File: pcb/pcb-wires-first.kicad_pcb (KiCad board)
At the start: 2 copper layers, 24 x 28.5 mm, 13 parts, among them J3 Conn_01x04, J4 Conn_01x06, SW1 SW_Push, SW2 SW_Push, U1 SLG47115V

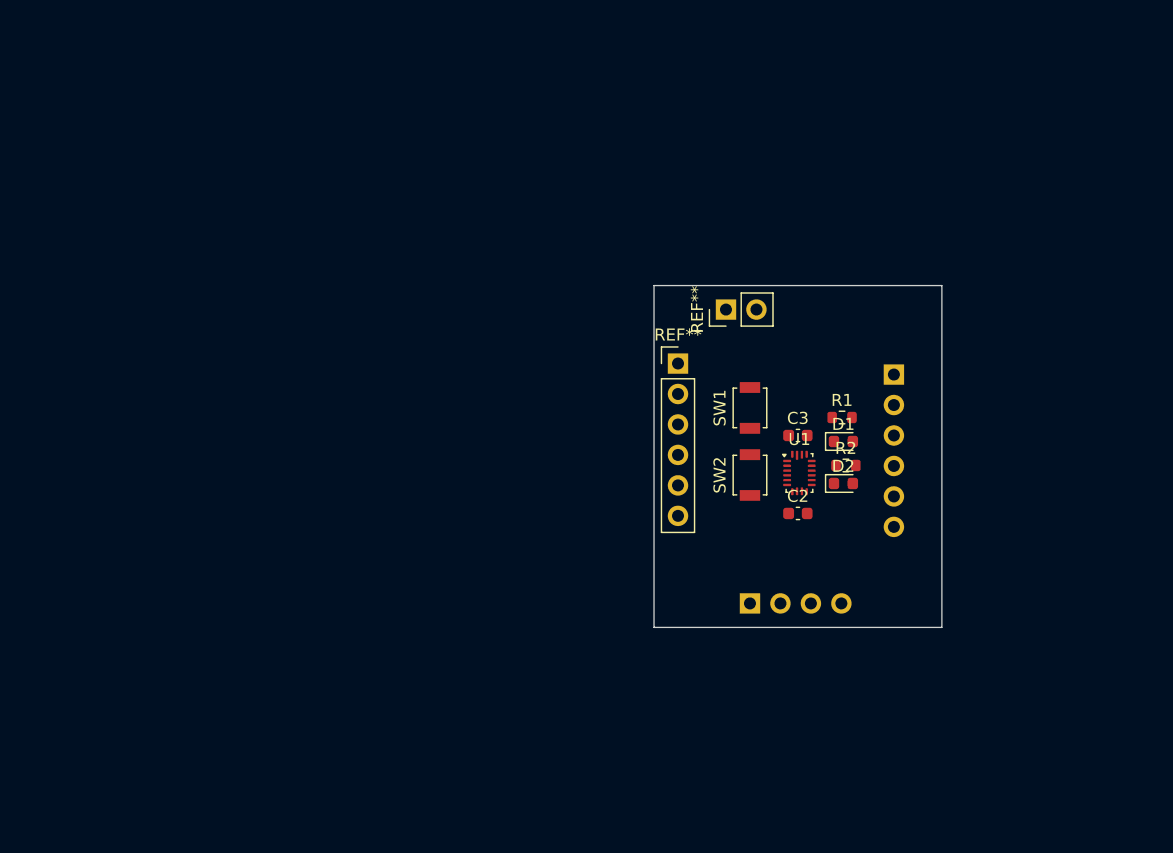
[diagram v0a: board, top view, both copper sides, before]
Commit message: Drafting the board.
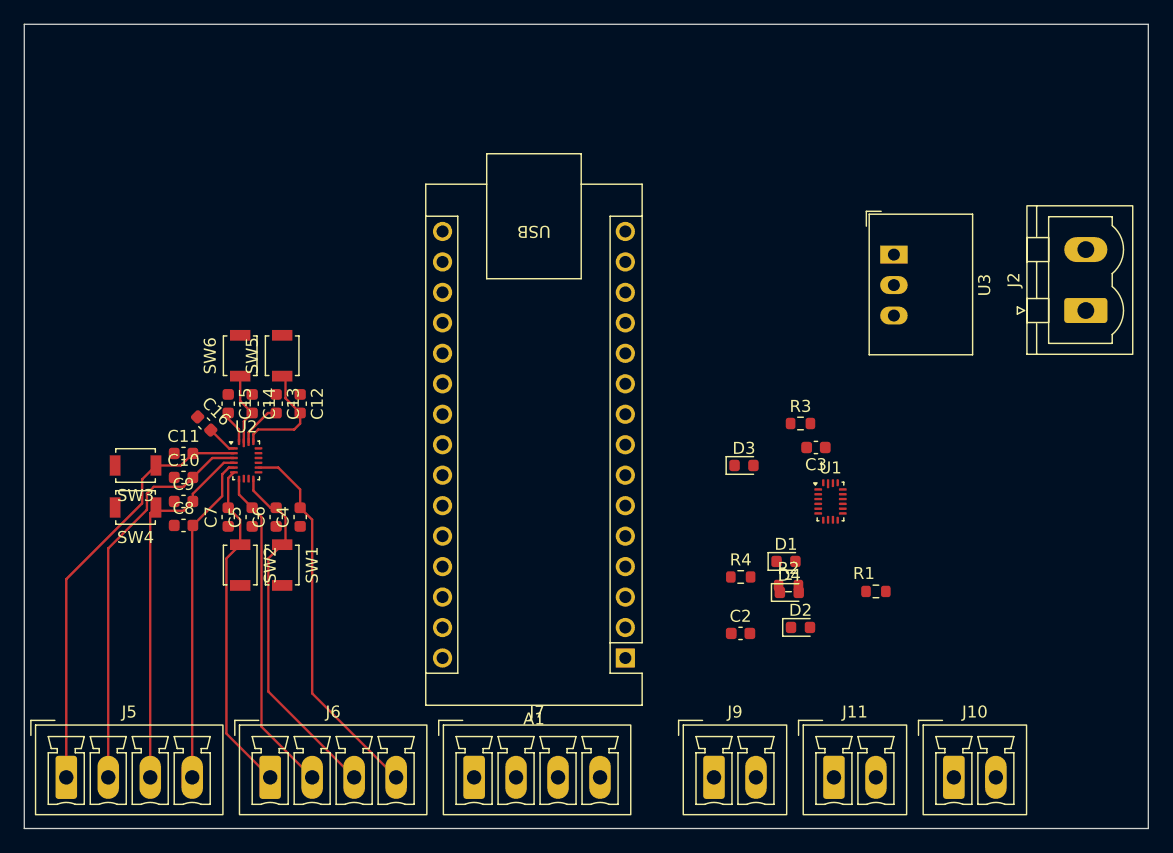
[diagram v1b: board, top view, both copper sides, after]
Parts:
- removed J3: Conn_01x04, Connector_PinHeader_2.54mm:PinHeader_1x04_P2.54mm_Vertical
- removed J4: Conn_01x06, Connector_PinHeader_2.54mm:PinHeader_1x06_P2.54mm_Vertical
- removed REF**: PinHeader_1x06_P2.54mm_Vertical, Connector_PinHeader_2.54mm:PinHeader_1x06_P2.54mm_Vertical
- removed REF**: PinHeader_1x02_P2.54mm_Vertical, Connector_PinHeader_2.54mm:PinHeader_1x02_P2.54mm_Vertical
- added A1: Arduino_Nano_ESP32, Module:Arduino_Nano, F.Cu at (95.6, 124.5)
- added C10: 100nF, Capacitor_SMD:C_0603_1608Metric, F.Cu at (58.8, 109.5)
- added C11: 100nF, Capacitor_SMD:C_0603_1608Metric, F.Cu at (58.8, 107.5)
- added C12: 100nF, Capacitor_SMD:C_0603_1608Metric, F.Cu at (68.5, 103.3)
- added C13: 100nF, Capacitor_SMD:C_0603_1608Metric, F.Cu at (66.5, 103.3)
- added C14: 100nF, Capacitor_SMD:C_0603_1608Metric, F.Cu at (64.5, 103.3)
- added C15: 100nF, Capacitor_SMD:C_0603_1608Metric, F.Cu at (62.5, 103.3)
- added C16: 100nF, Capacitor_SMD:C_0603_1608Metric, F.Cu at (60.5, 105.0)
- added C4: 100nF, Capacitor_SMD:C_0603_1608Metric, F.Cu at (68.5, 112.8)
- added C5: 100nF, Capacitor_SMD:C_0603_1608Metric, F.Cu at (64.5, 112.8)
- added C6: 100nF, Capacitor_SMD:C_0603_1608Metric, F.Cu at (66.5, 112.8)
- added C7: 100nF, Capacitor_SMD:C_0603_1608Metric, F.Cu at (62.5, 112.8)
- added C8: 100nF, Capacitor_SMD:C_0603_1608Metric, F.Cu at (58.8, 113.5)
- added C9: 100nF, Capacitor_SMD:C_0603_1608Metric, F.Cu at (58.8, 111.5)
- added D3: ON, Diode_SMD:D_0603_1608Metric, F.Cu at (105.5, 108.5)
- added D4: ON, Diode_SMD:D_0603_1608Metric, F.Cu at (109.3, 119.1)
- added J10: Conn_01x02, Connector_Phoenix_MC:PhoenixContact_MCV_1,5_2-G-3.5_1x02_P3.50mm_Vertical, F.Cu at (123.0, 134.5)
- added J11: Conn_01x02, Connector_Phoenix_MC:PhoenixContact_MCV_1,5_2-G-3.5_1x02_P3.50mm_Vertical, F.Cu at (113.0, 134.5)
- added J2: Conn_01x02, Connector_Phoenix_MSTB:PhoenixContact_MSTBVA_2,5_2-G-5,08_1x02_P5.08mm_Vertical, F.Cu at (134.0, 95.6)
- added J5: Conn_01x04, Connector_Phoenix_MC:PhoenixContact_MCV_1,5_4-G-3.5_1x04_P3.50mm_Vertical, F.Cu at (49.0, 134.5)
- added J6: Conn_01x04, Connector_Phoenix_MC:PhoenixContact_MCV_1,5_4-G-3.5_1x04_P3.50mm_Vertical, F.Cu at (66.0, 134.5)
- added J7: Conn_01x04, Connector_Phoenix_MC:PhoenixContact_MCV_1,5_4-G-3.5_1x04_P3.50mm_Vertical, F.Cu at (83.0, 134.5)
- added J9: Conn_01x02, Connector_Phoenix_MC:PhoenixContact_MCV_1,5_2-G-3.5_1x02_P3.50mm_Vertical, F.Cu at (103.0, 134.5)
- added R3: 510, Resistor_SMD:R_0603_1608Metric, F.Cu at (110.2, 105.0)
- added R4: 510, Resistor_SMD:R_0603_1608Metric, F.Cu at (105.2, 117.8)
- added SW3: on-1, Button_Switch_SMD:SW_SPST_B3U-1000P, F.Cu at (54.8, 108.5)
- added SW4: off-1, Button_Switch_SMD:SW_SPST_B3U-1000P, F.Cu at (54.8, 112.0)
- added SW5: on-3, Button_Switch_SMD:SW_SPST_B3U-1000P, F.Cu at (67.0, 99.3)
- added SW6: off-3, Button_Switch_SMD:SW_SPST_B3U-1000P, F.Cu at (63.5, 99.3)
- added U2: SLG46826V, Package_DFN_QFN:Renesas_UQFN-20_2x3mm_P0.4mm_LayoutBorder4x6y, F.Cu at (64.0, 108.1)
- added U3: R-78C3.3-1.0, Converter_DCDC:Converter_DCDC_RECOM_R-78E-0.5_THT, F.Cu at (118.0, 90.9)
- SW1: value SW_Push -> off-2
- SW2: value SW_Push -> on-2
- moved SW2 43.2 mm to (63.5, 116.8), turned to -90 degrees
- moved SW1 41.1 mm to (67.0, 116.8), turned to -90 degrees
- moved R1 14.8 mm to (116.5, 119.0)
- moved D2 12.5 mm to (110.2, 122.0)
- moved C2 11.1 mm to (105.2, 122.5)
- moved D1 11.1 mm to (109.0, 116.5)
- moved R2 11.1 mm to (109.2, 118.5)
- moved U1 3.51 mm to (112.7, 111.5)
- moved C3 1.80 mm to (111.5, 107.0), turned to 180 degrees
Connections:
- C2 pad 1: HV_GND -> GND
- D2 pad 1: GND -> unconnected-(D2-K-Pad1)
- R1 pad 1: Net-(J4-Pin_3) -> Net-(A1-A2)
- R2 pad 1: Net-(J4-Pin_2) -> unconnected-(R2-Pad1)
- SW1 pad 1: GND -> /off-2a
- SW1 pad 2: /turn-off-sw -> GND
- SW2 pad 1: GND -> /on-2a
- SW2 pad 2: /turn-on-sw -> GND
- U1 pad 10: Net-(J3-Pin_3) -> unconnected-(U1-HV_GPO3-Pad10)
- U1 pad 13: HV_GND -> GND
- U1 pad 14: Net-(J4-Pin_2) -> Net-(A1-A1)
- U1 pad 15: Net-(J4-Pin_5) -> unconnected-(U1-SCL-Pad15)
- U1 pad 16: Net-(J4-Pin_4) -> unconnected-(U1-SDA-Pad16)
- U1 pad 17: Net-(J4-Pin_3) -> Net-(A1-A0)
- U1 pad 19: /turn-on-hw -> unconnected-(U1-GPIO5-Pad19)
- U1 pad 2: /turn-off-sw -> Net-(A1-A2)
- U1 pad 20: /turn-on-sw -> unconnected-(U1-GPIO6-Pad20)
- U1 pad 3: /turn-off-hw -> unconnected-(U1-GPI-Pad3)
- U1 pad 4: HV_GND -> GND
- U1 pad 7: Net-(J3-Pin_2) -> Net-(J11-Pin_2)
- U1 pad 8: Net-(J3-Pin_2) -> Net-(J10-Pin_2)
- U1 pad 9: Net-(J3-Pin_3) -> Net-(J9-Pin_2)
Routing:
- net /on-1a: track 0.00 -> 36.0 mm
- net /on-1b: track 0.00 -> 33.5 mm
- net /off-2b: track 0.00 -> 31.5 mm
- net /off-1a: track 0.00 -> 31.3 mm
- net /off-2a: track 0.00 -> 29.8 mm
- net /on-2a: track 0.00 -> 28.0 mm
- net /off-1b: track 0.00 -> 27.5 mm
- net /on-2b: track 0.00 -> 27.4 mm
- net /on-3a: track 0.00 -> 9.46 mm
- net /off-3a: track 0.00 -> 6.25 mm
- net /on-3b: track 0.00 -> 3.78 mm
- net /off-3b: track 0.00 -> 2.76 mm
- net VDD: track 0.00 -> 2.56 mm
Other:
- board size 24 x 28.5 mm -> 93.7 x 67 mm
